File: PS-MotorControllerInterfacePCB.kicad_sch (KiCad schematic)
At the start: 49 parts, among them J1 53307-2471, J2 MotorController-in, J3 Conn_01x06, J4 PEAK, J6 MotorController-out, U2 MCP16331x-xCH

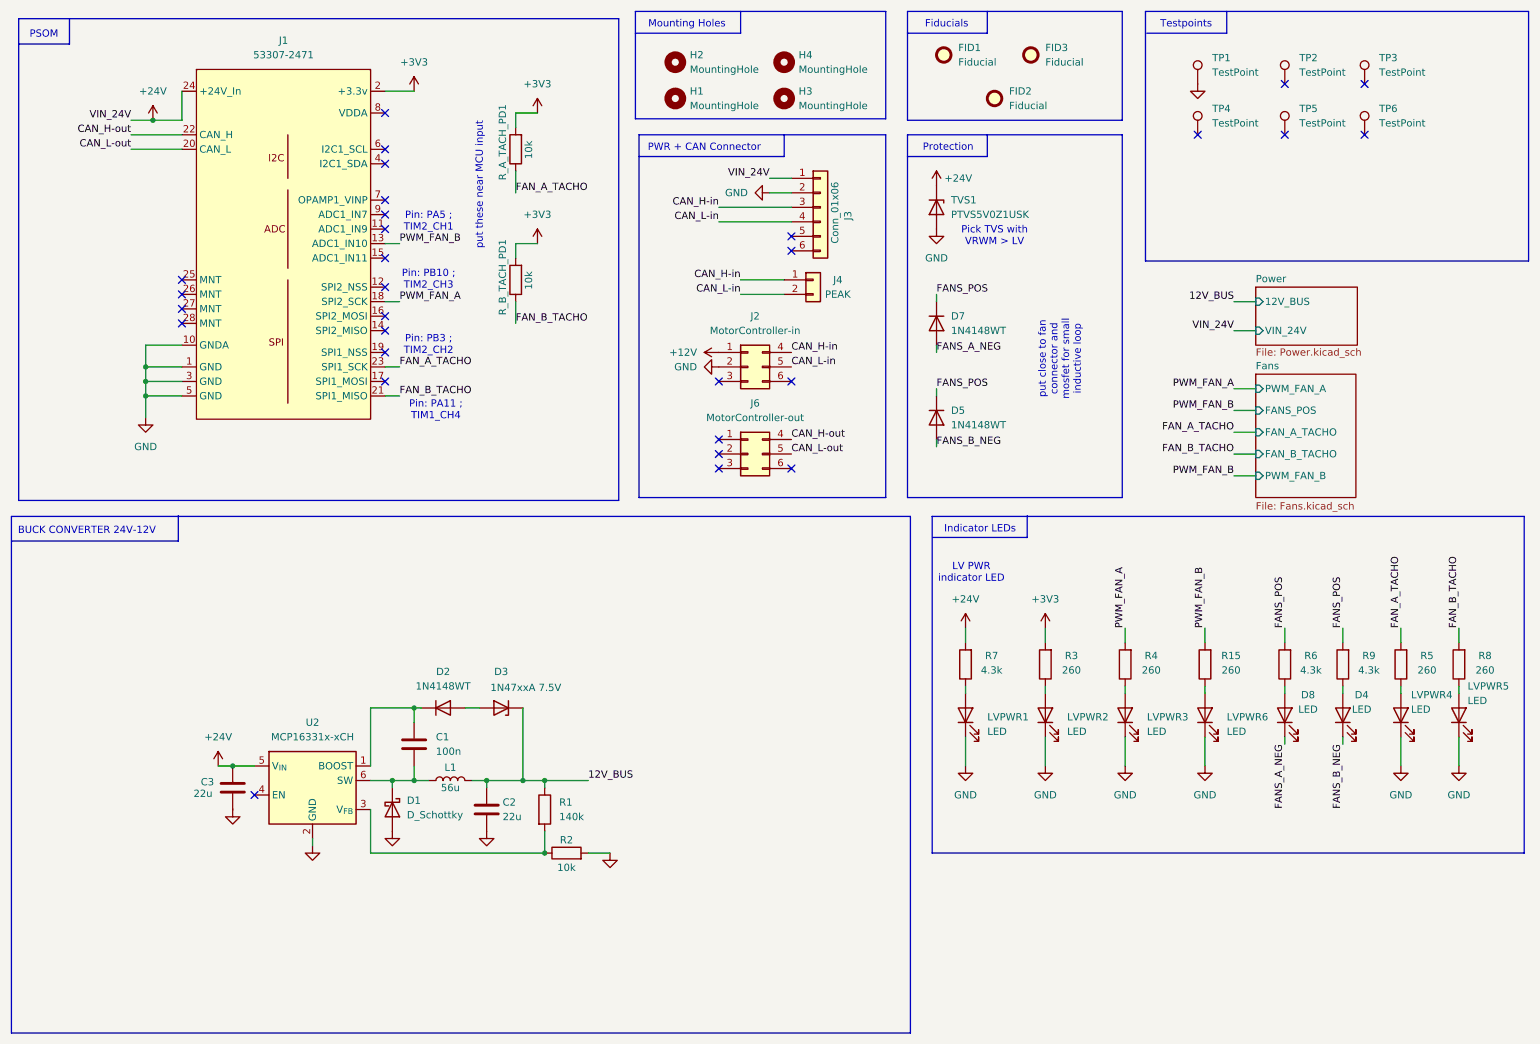
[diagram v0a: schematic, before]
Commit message: schematic
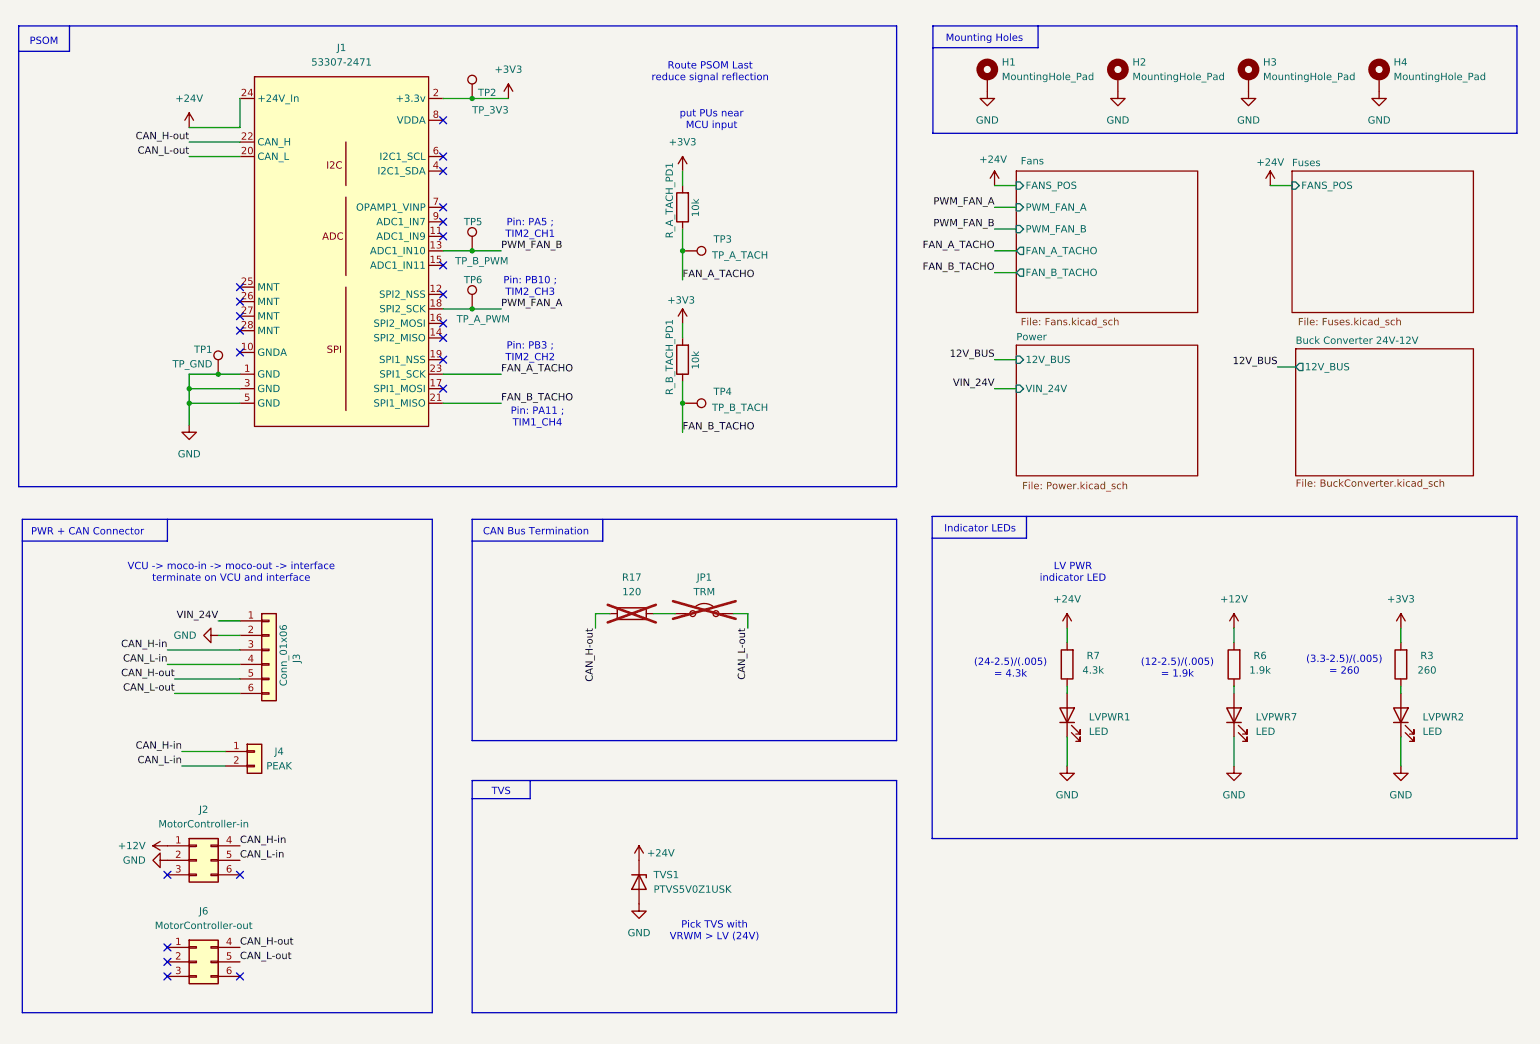
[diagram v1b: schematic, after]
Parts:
- removed C1: 100n, symbol Device:C
- removed C2, C3: 22u, symbol Device:C
- removed D1: D_Schottky, symbol Device:D_Schottky
- removed D2, D5, D7: 1N4148WT, Diode_SMD:D_SOD-523, symbol Diode:1N4148WT
- removed D3: 1N47xxA 7.5V, Diode_THT:D_DO-41_SOD81_P10.16mm_Horizontal, symbol Diode:1N47xxA
- removed D4, D8: LED, symbol Device:LED
- removed FID1, FID2, FID3: Fiducial, symbol Mechanical:Fiducial
- removed H1, H2, H3, H4: MountingHole, symbol Mechanical:MountingHole
- removed L1: 56u, symbol Device:L
- removed LVPWR3, LVPWR4, LVPWR5, LVPWR6: LED, LED_SMD:LED_0603_1608Metric, symbol Device:LED
- removed R1: 140k, symbol Device:R
- removed R15, R4, R5, R8: 260, symbol Device:R
- removed R2: 10k, symbol Device:R
- removed R9: 4.3k, symbol Device:R
- removed U2: MCP16331x-xCH, Package_TO_SOT_SMD:SOT-23-6, symbol Regulator_Switching:MCP16331x-xCH
- added H1, H2, H3, H4: MountingHole_Pad, symbol Mechanical:MountingHole_Pad
- added JP1: TRM, Connector_PinHeader_2.54mm:PinHeader_1x02_P2.54mm_Vertical, symbol Jumper:Jumper_2_Open
- added LVPWR7: LED, LED_SMD:LED_0603_1608Metric, symbol Device:LED
- added R17: 120, Resistor_SMD:R_0603_1608Metric_Pad0.98x0.95mm_HandSolder, symbol Device:R
- R6: value 4.3k -> 1.9k
- TP1: value TestPoint -> TP_GND
- TP2: value TestPoint -> TP_3V3
- TP3: value TestPoint -> TP_A_TACH
- TP4: value TestPoint -> TP_B_TACH
- TP5: value TestPoint -> TP_B_PWM
- TP6: value TestPoint -> TP_A_PWM
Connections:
- net FANS_POS is gone; now on net +12V: R6.2
- net +24V: no longer J3.1 (Pin_1)
- net +3V3: now also TP2.1
- net CAN_H-out: now also J3.5 (Pin_5), R17.1
- net CAN_L-out: now also J3.6 (Pin_6), JP1.2 (B)
- net FAN_A_TACHO: now also TP3.1
- net FAN_B_TACHO: now also TP4.1
- net GND: now also H1.1, H2.1, H3.1, H4.1, LVPWR7.1 (K); no longer J1.10 (GNDA)
- net PWM_FAN_A: now also TP6.1
- net PWM_FAN_B: now also TP5.1
- net at R6.1: now also LVPWR7.2 (A)
- new net: JP1.1 (A), R17.2
- new net VIN_24V: J3.1 (Pin_1)
- no-connect marks 30 -> 23
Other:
- added sheet Buck Converter 24V-12V (BuckConverter.kicad_sch)
- added sheet Fuses (Fuses.kicad_sch)
- note added: "(12-2.5)/(.005) = 1.9k"
- note added: "(24-2.5)/(.005) = 4.3k"
- note added: "(3.3-2.5)/(.005) = 260"
- note added: "CAN Bus Termination"
- note added: "Pick TVS with VRWM > LV (24V)"
- note added: "Route PSOM Last reduce signal reflection"
- note added: "TVS"
- note added: "VCU -> moco-in -> moco-out -> interface terminate on VCU and interface"
- note added: "put PUs near MCU input"
- note removed: "BUCK CONVERTER 24V-12V"
- note removed: "Fiducials"
- note removed: "Pick TVS with VRWM > LV"
- note removed: "Protection"
- note removed: "Testpoints"
- note removed: "put close to fan connector and mosfet for small inductive loop"
- note removed: "put these near MCU input"
- moved on the sheet: J1, J2, J3, J4, J6, LVPWR1, LVPWR2, R3, R7, R_A_TACH_PD1, R_B_TACH_PD1, TVS1
